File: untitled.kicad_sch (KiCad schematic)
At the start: 60 parts, among them J1 Conn_01x04_Pin, J10 Conn_01x03_Pin, J2 USB_B_Micro, J3 Conn_01x02_Pin, J4 Conn_01x02_Pin, J6 Screw_Terminal_01x02, J9 Screw_Terminal_01x02, U1 STM32F767ZITx, U2 MAX17501AATB+, U5 AT24C256, U8 AMS1117-3.3, Y1 16MHz

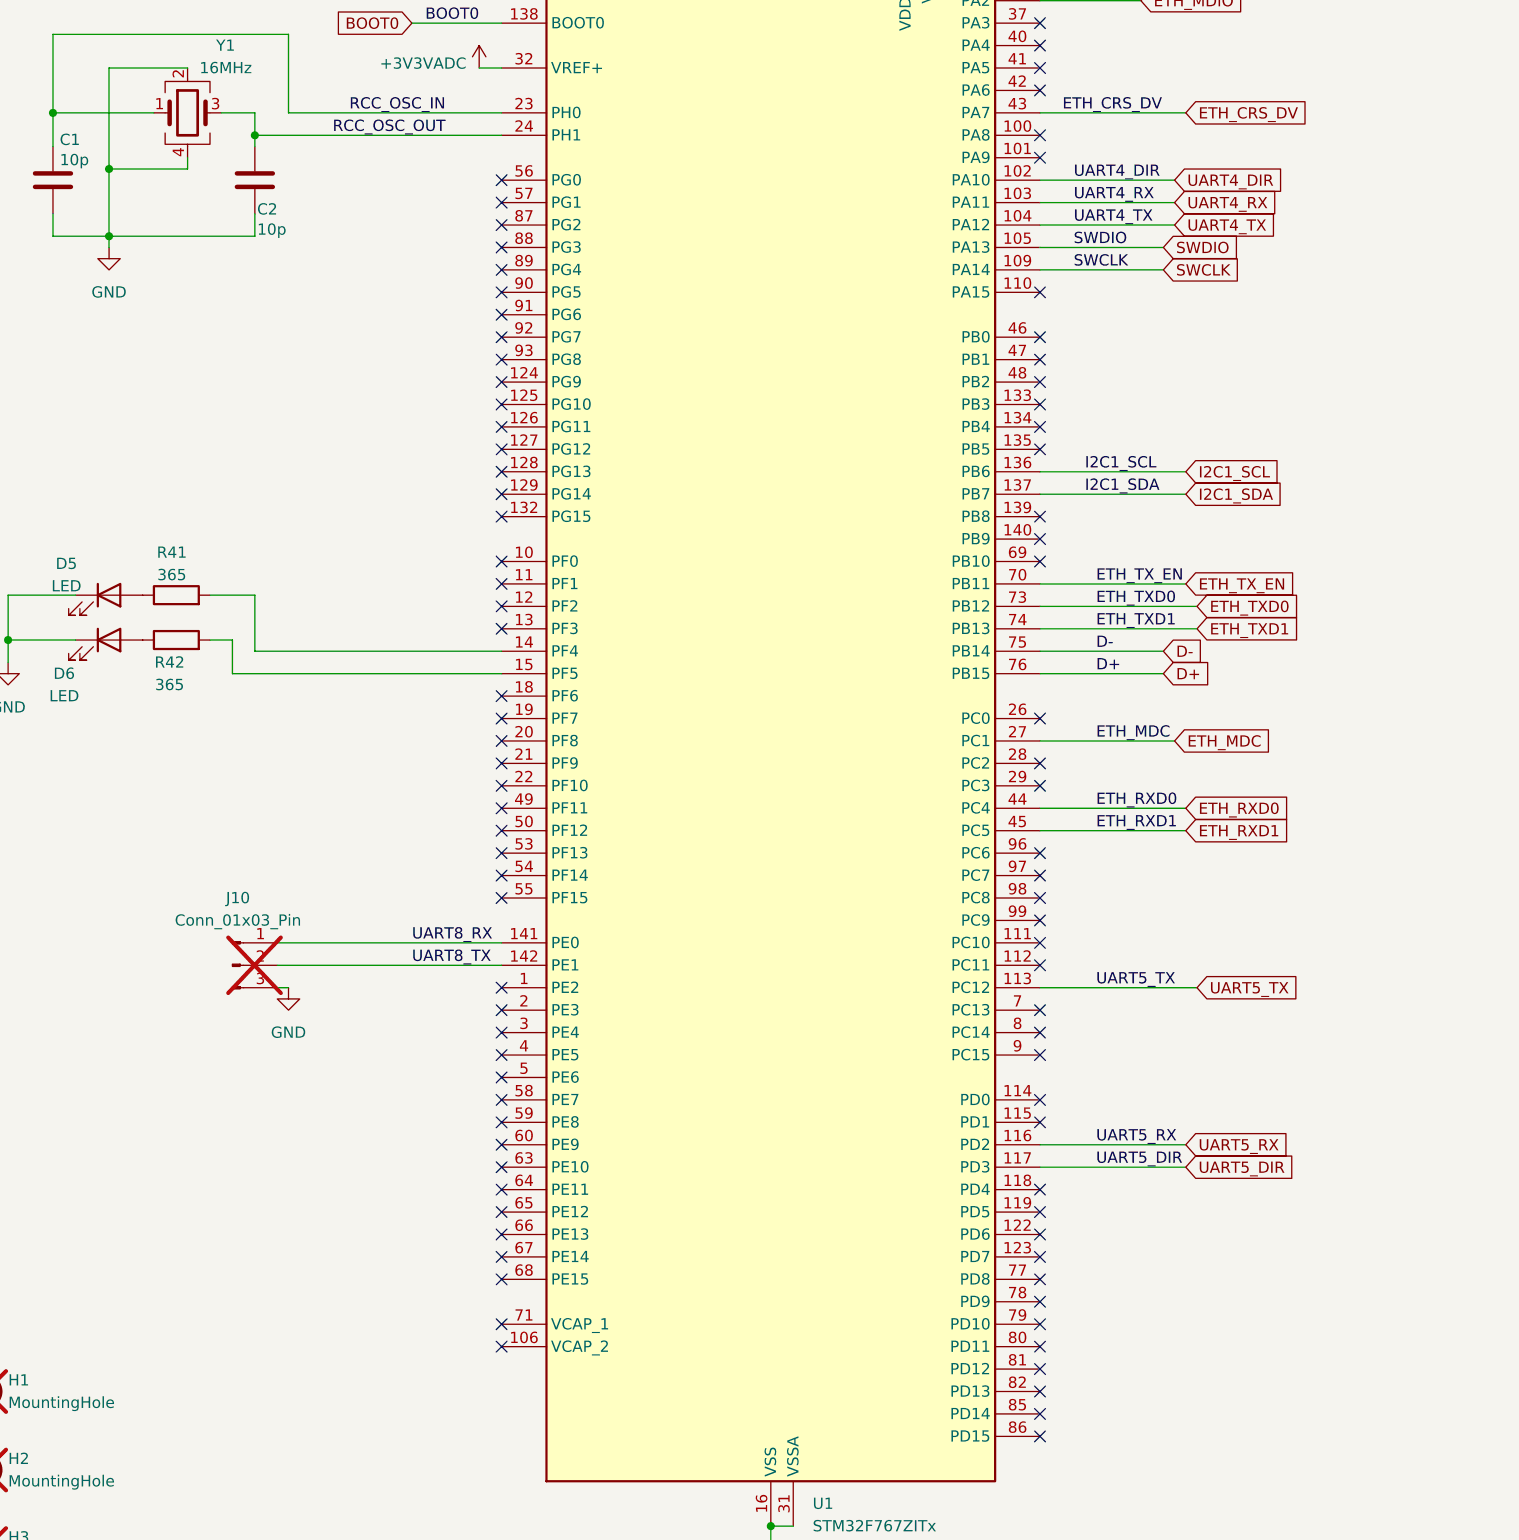
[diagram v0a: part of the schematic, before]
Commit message: SCH Save: 1 files changed untitled.kicad_sch 0/10/205
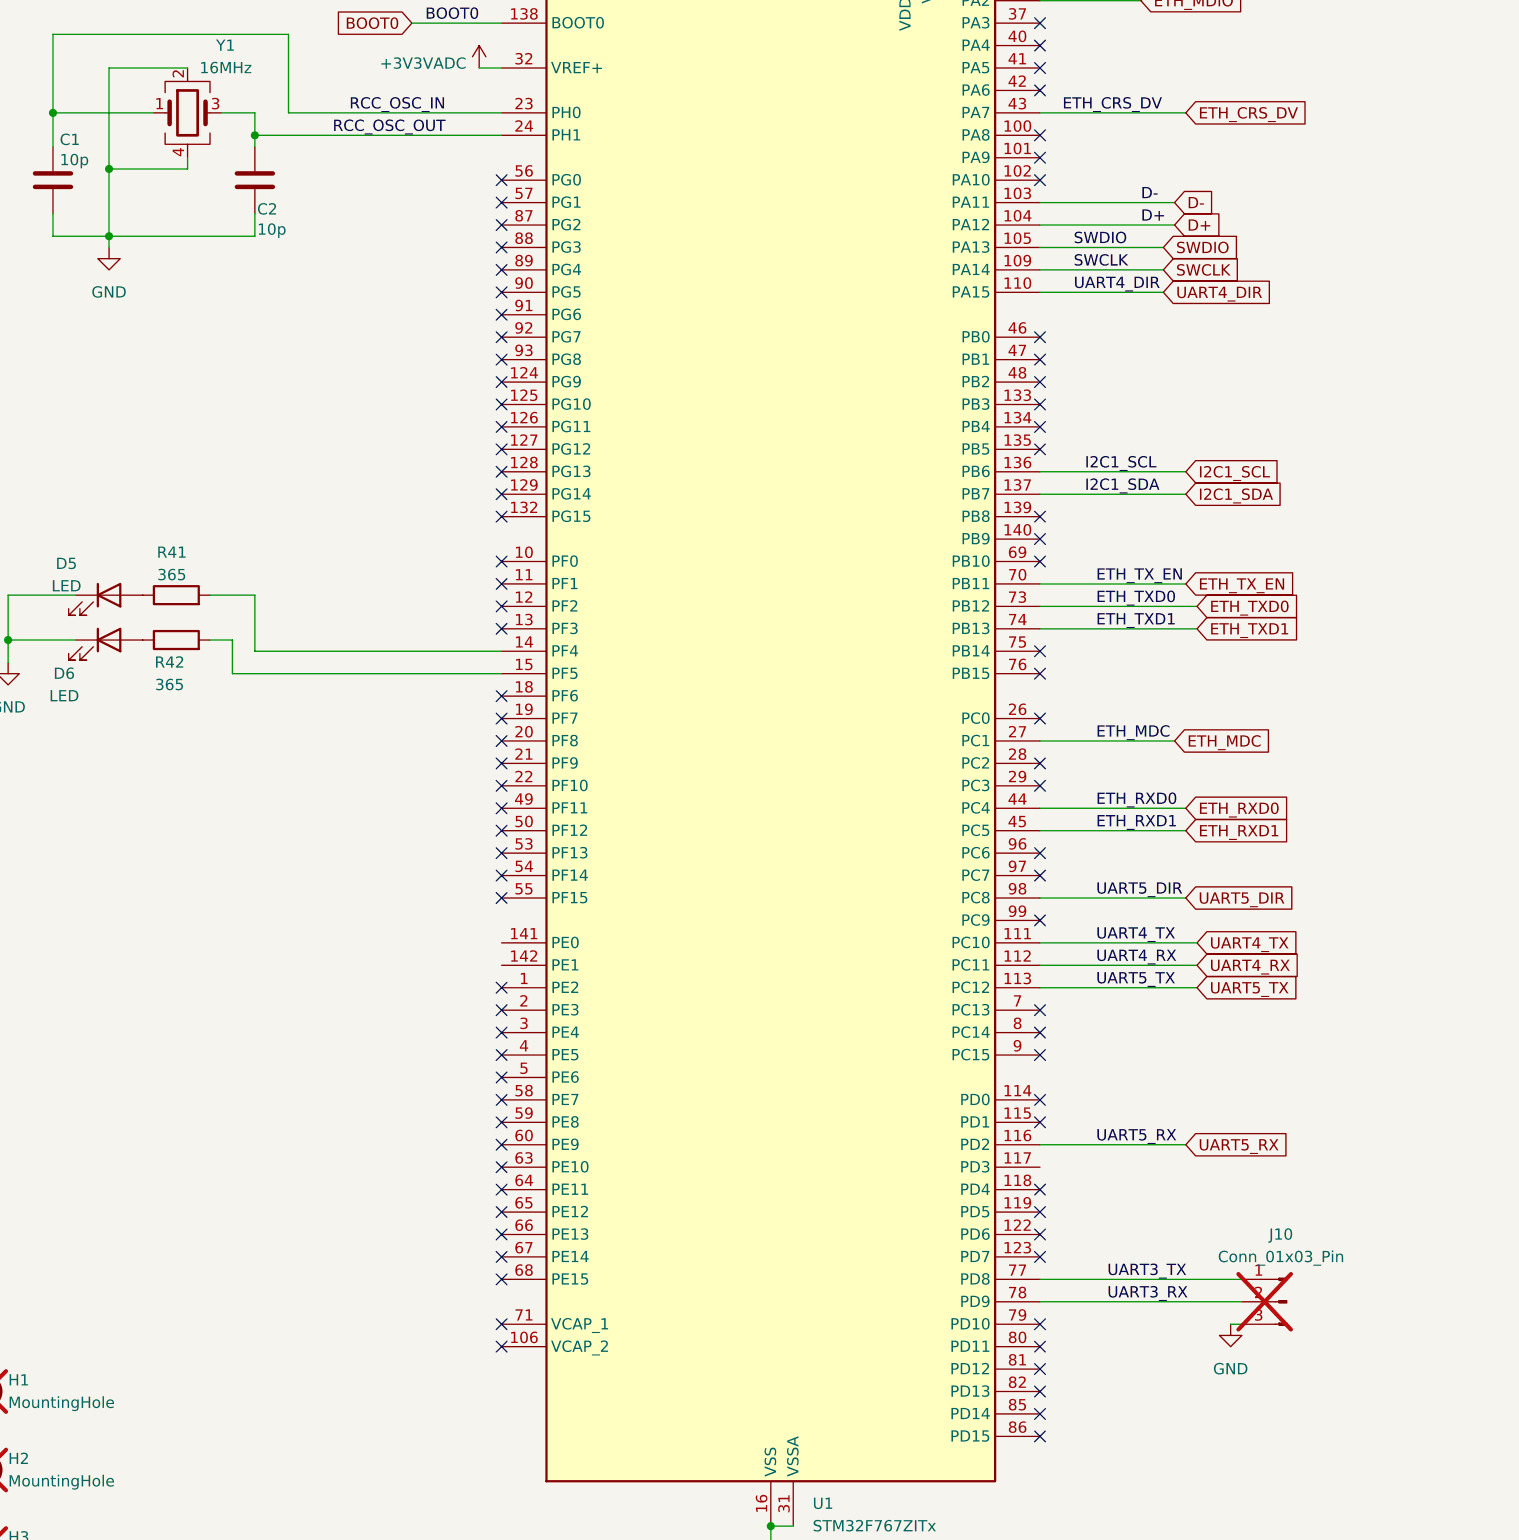
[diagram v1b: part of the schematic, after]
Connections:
- net D+: now also U1.104 (PA12); no longer U1.76 (PB15)
- net D-: now also U1.103 (PA11); no longer U1.75 (PB14)
- net UART4_DIR: now also U1.110 (PA15); no longer U1.102 (PA10)
- net UART4_RX: now also U1.112 (PC11); no longer U1.103 (PA11)
- net UART4_TX: now also U1.111 (PC10); no longer U1.104 (PA12)
- net UART5_DIR: now also U1.98 (PC8); no longer U1.117 (PD3)
- net UART3_TX: now reaches U1.77 (PD8)
- net UART3_TX: now also J10.1 (Pin_1)
- net UART3_RX: now reaches U1.78 (PD9)
- net UART3_RX: now also J10.2 (Pin_2)
- net UART8_RX: no longer names the net of U1.141 (PE0)
- net UART8_RX: no longer J10.1 (Pin_1)
- net UART8_TX: no longer names the net of U1.142 (PE1)
- net UART8_TX: no longer J10.2 (Pin_2)
- no-connect marks 96 -> 93
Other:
- moved on the sheet: J10
